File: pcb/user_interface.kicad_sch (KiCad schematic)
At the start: 5 parts

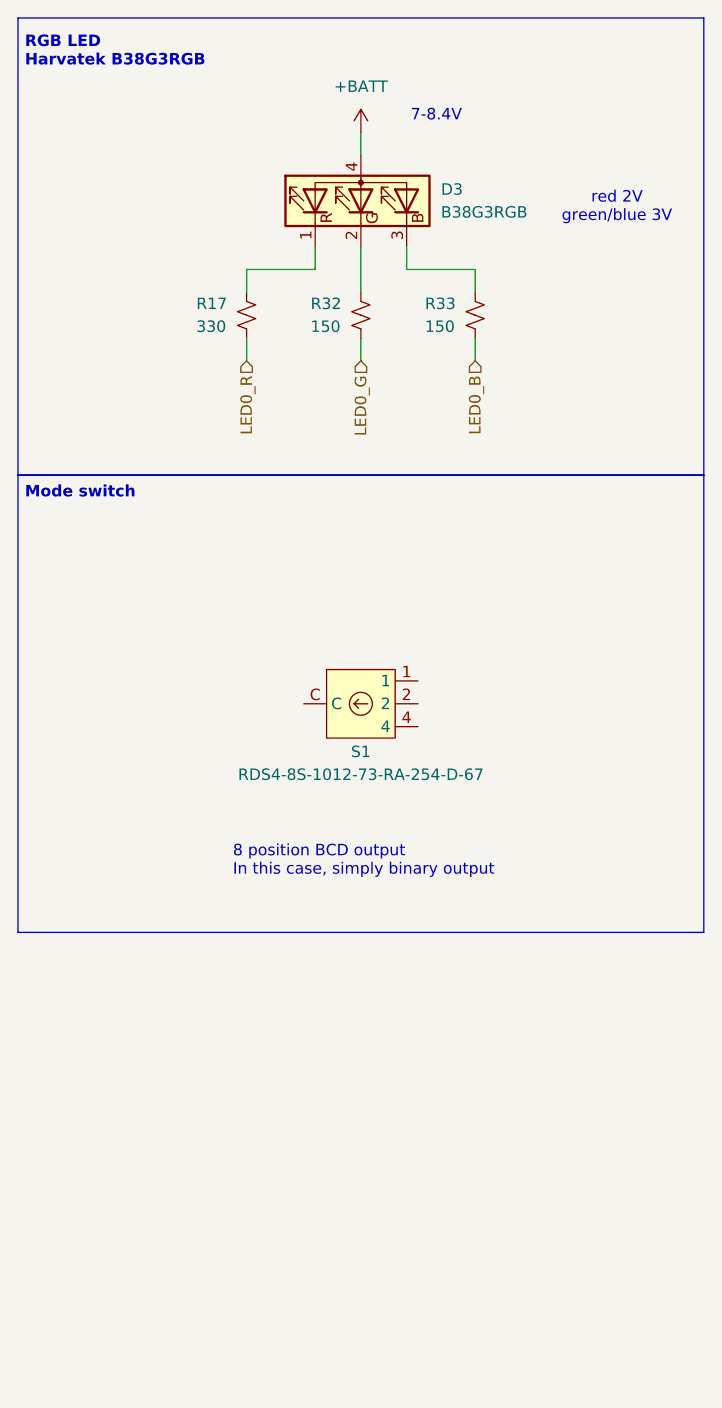
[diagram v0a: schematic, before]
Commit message: Add buzzer symbol to user interface
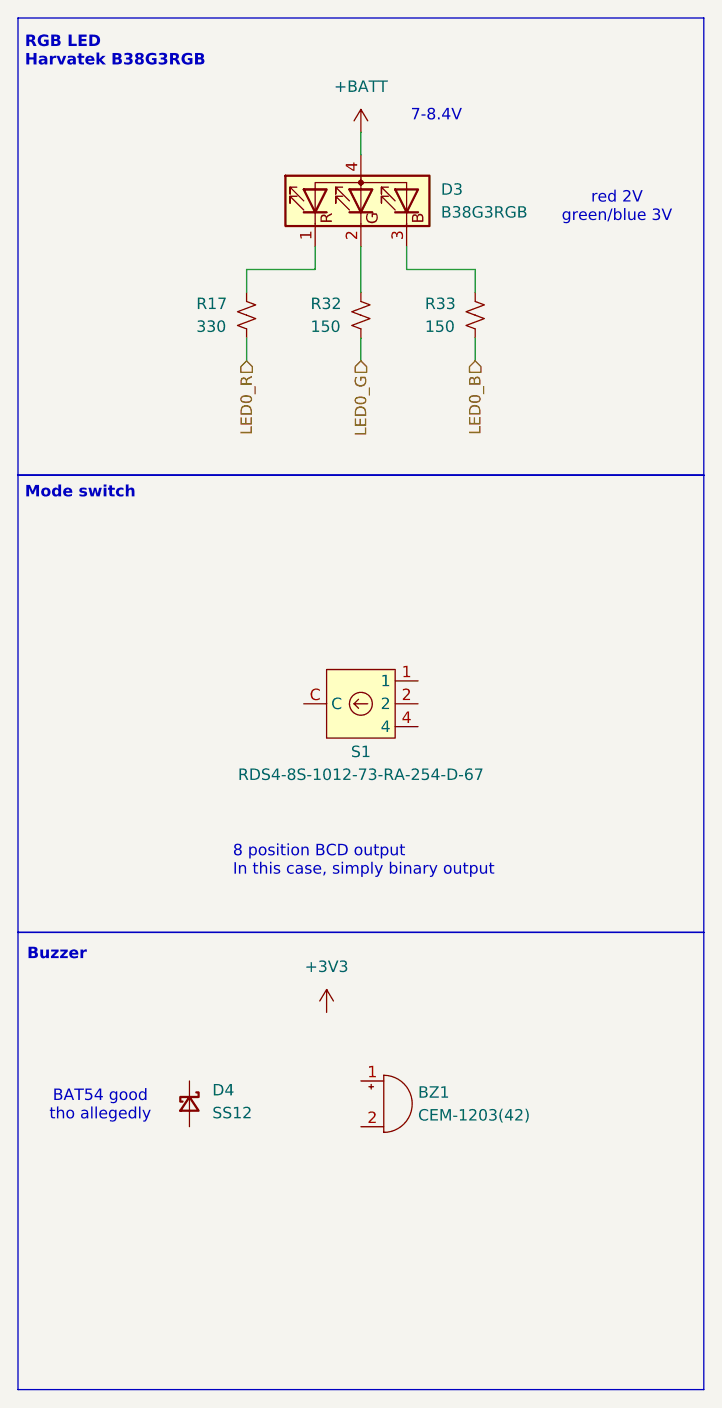
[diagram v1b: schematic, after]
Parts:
- added BZ1: CEM-1203(42), Buzzer_SameSky:Buzzer_SameSky_CEM-1203_42, symbol Device:Buzzer
- added D4: SS12, symbol Device:D_Schottky_Small
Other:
- note added: "BAT54 good tho allegedly"
- note added: "Buzzer"
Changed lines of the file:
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@@
+	)
+	(rectangle
+		(start 12.7 114.3)
+		(end 88.9 165.1)
+		(stroke
+			(width 0)
+			(type default)
+		)
+		(fill
+			(type none)
+		)
 	)
 	(rectangle
@@
 		)
 	)
+	(text "Buzzer"
+		(exclude_from_sim no)
+		(at 13.716 116.078 0)
+		(effects
+			(font
+				(size 1.27 1.27)
+				(thickness 0.254)
+				(bold yes)
+			)
+			(justify left top)
+		)
+	)
 	(text "red 2V\ngreen/blue 3V"
 		(exclude_from_sim no)
 		(at 79.248 33.782 0)
+		(effects
+			(font
+				(size 1.27 1.27)
+			)
+		)
+	)
+	(text "BAT54 good\ntho allegedly"
+		(exclude_from_sim no)
+		(at 21.844 133.604 0)
 		(effects
 			(font
@@
 			)
 			(justify right)
+		)
+	)
+	(symbol
+		(lib_id "Device:Buzzer")
+		(at 53.34 133.35 0)
+		(unit 1)
+		(exclude_from_sim no)
+		(in_bom yes)
+		(on_board yes)
+		(dnp no)
+		(fields_autoplaced yes)
+		(property "Reference" "BZ1"
+			(at 57.15 132.0799 0)
+			(effects
+				(font
+					(size 1.27 1.27)
+				)
+				(justify left)
+			)
+		)
+		(property "Value" "CEM-1203(42)"
+			(at 57.15 134.6199 0)
+			(effects
+				(font
+					(size 1.27 1.27)
+				)
+				(justify left)
+			)
+		)
+		(property "Footprint" "Buzzer_SameSky:Buzzer_SameSky_CEM-1203_42"
+			(at 52.705 130.81 90)
+			(effects
+				(font
+					(size 1.27 1.27)
+				)
+				(hide yes)
+			)
+		)
+		(property "Datasheet" "~"
+			(at 52.705 130.81 90)
+			(effects
+				(font
+					(size 1.27 1.27)
+				)
+				(hide yes)
+			)
+		)
+		(property "Description" "Buzzer, polarized"
+			(at 53.34 133.35 0)
+			(effects
+				(font
+					(size 1.27 1.27)
+				)
+				(hide yes)
+			)
+		)
+		(pin "1"
+		)
+		(pin "2"
+		)
+		(instances
+			(project ""
+				(path "/1f4fd4ed-9886-4375-a5ac-dc32d5760936/0a32b07f-7988-40ae-8006-b298a5ae2a50"
+					(reference "BZ1")
+					(unit 1)
+				)
+			)
 		)
 	)
@@
 					(unit 1)
 				)
+			)
+		)
+	)
+	(symbol
+		(lib_id "Device:D_Schottky_Small")
+		(at 31.75 133.35 270)
+		(unit 1)
+		(exclude_from_sim no)
+		(in_bom yes)
+		(on_board yes)
+		(dnp no)
+		(fields_autoplaced yes)
+		(property "Reference" "D4"
+			(at 34.29 131.8259 90)
+			(effects
+				(font
+					(size 1.27 1.27)
+				)
+				(justify left)
+			)
+		)
+		(property "Value" "SS12"
+			(at 34.29 134.3659 90)
+			(effects
+				(font
+					(size 1.27 1.27)
+				)
+				(justify left)
+			)
+		)
+		(property "Footprint" ""
+			(at 31.75 133.35 90)
+			(effects
+				(font
+					(size 1.27 1.27)
+				)
+				(hide yes)
+			)
+		)
+		(property "Datasheet" "~"
+			(at 31.75 133.35 90)
+			(effects
+				(font
+					(size 1.27 1.27)
+				)
+				(hide yes)
+			)
+		)
+		(property "Description" "Schottky diode, small symbol"
+			(at 31.75 133.35 0)
+			(effects
+				(font
+					(size 1.27 1.27)
+				)
+				(hide yes)
+			)
+		)
+		(pin "2"
+		)
+		(pin "1"
+		)
+		(instances
+			(project ""
+				(path "/1f4fd4ed-9886-4375-a5ac-dc32d5760936/0a32b07f-7988-40ae-8006-b298a5ae2a50"
+					(reference "D4")
+					(unit 1)
+				)
+			)
+		)
+	)
+	(symbol
+		(lib_id "power:+3V3")
+		(at 46.99 123.19 0)
+		(unit 1)
+		(exclude_from_sim no)
+		(in_bom yes)
+		(on_board yes)
+		(dnp no)
+		(fields_autoplaced yes)
+		(property "Reference" "#PWR069"
+			(at 46.99 127 0)
+			(effects
+				(font
+					(size 1.27 1.27)
+				)
+				(hide yes)
+			)
+		)
+		(property "Value" "+3V3"
+			(at 46.99 118.11 0)
+			(effects
+				(font
+					(size 1.27 1.27)
+				)
+			)
+		)
+		(property "Footprint" ""
+			(at 46.99 123.19 0)
+			(effects
+				(font
+					(size 1.27 1.27)
+				)
+				(hide yes)
+			)
+		)
+		(property "Datasheet" ""
+			(at 46.99 123.19 0)
+			(effects
+				(font
+					(size 1.27 1.27)
+				)
+				(hide yes)
+			)
+		)
+		(property "Description" "Power symbol creates a global label with name \"+3V3\""
+			(at 46.99 123.19 0)
+			(effects
+				(font
+					(size 1.27 1.27)
+				)
+				(hide yes)
+			)
+		)
+		(pin "1"
+		)
+		(instances
+			(project ""
+				(path "/1f4fd4ed-9886-4375-a5ac-dc32d5760936/0a32b07f-7988-40ae-8006-b298a5ae2a50"
+					(reference "#PWR069")
+					(unit 1)
+				)
